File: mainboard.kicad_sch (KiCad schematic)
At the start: 0 parts

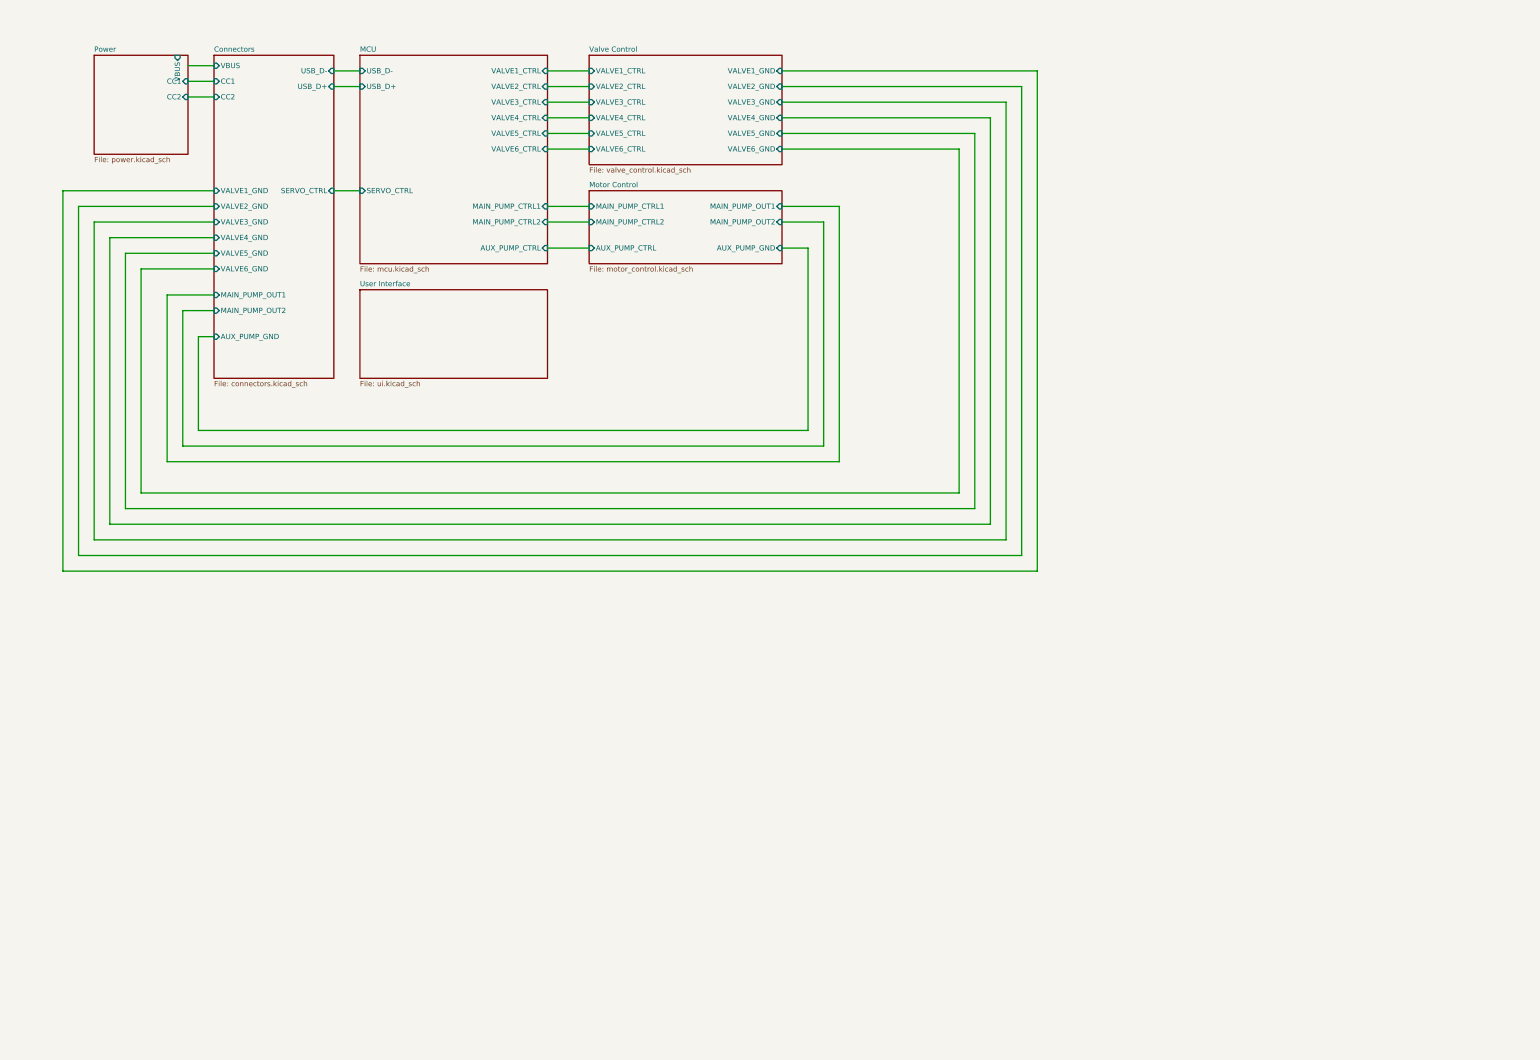
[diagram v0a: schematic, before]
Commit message: Finish first design
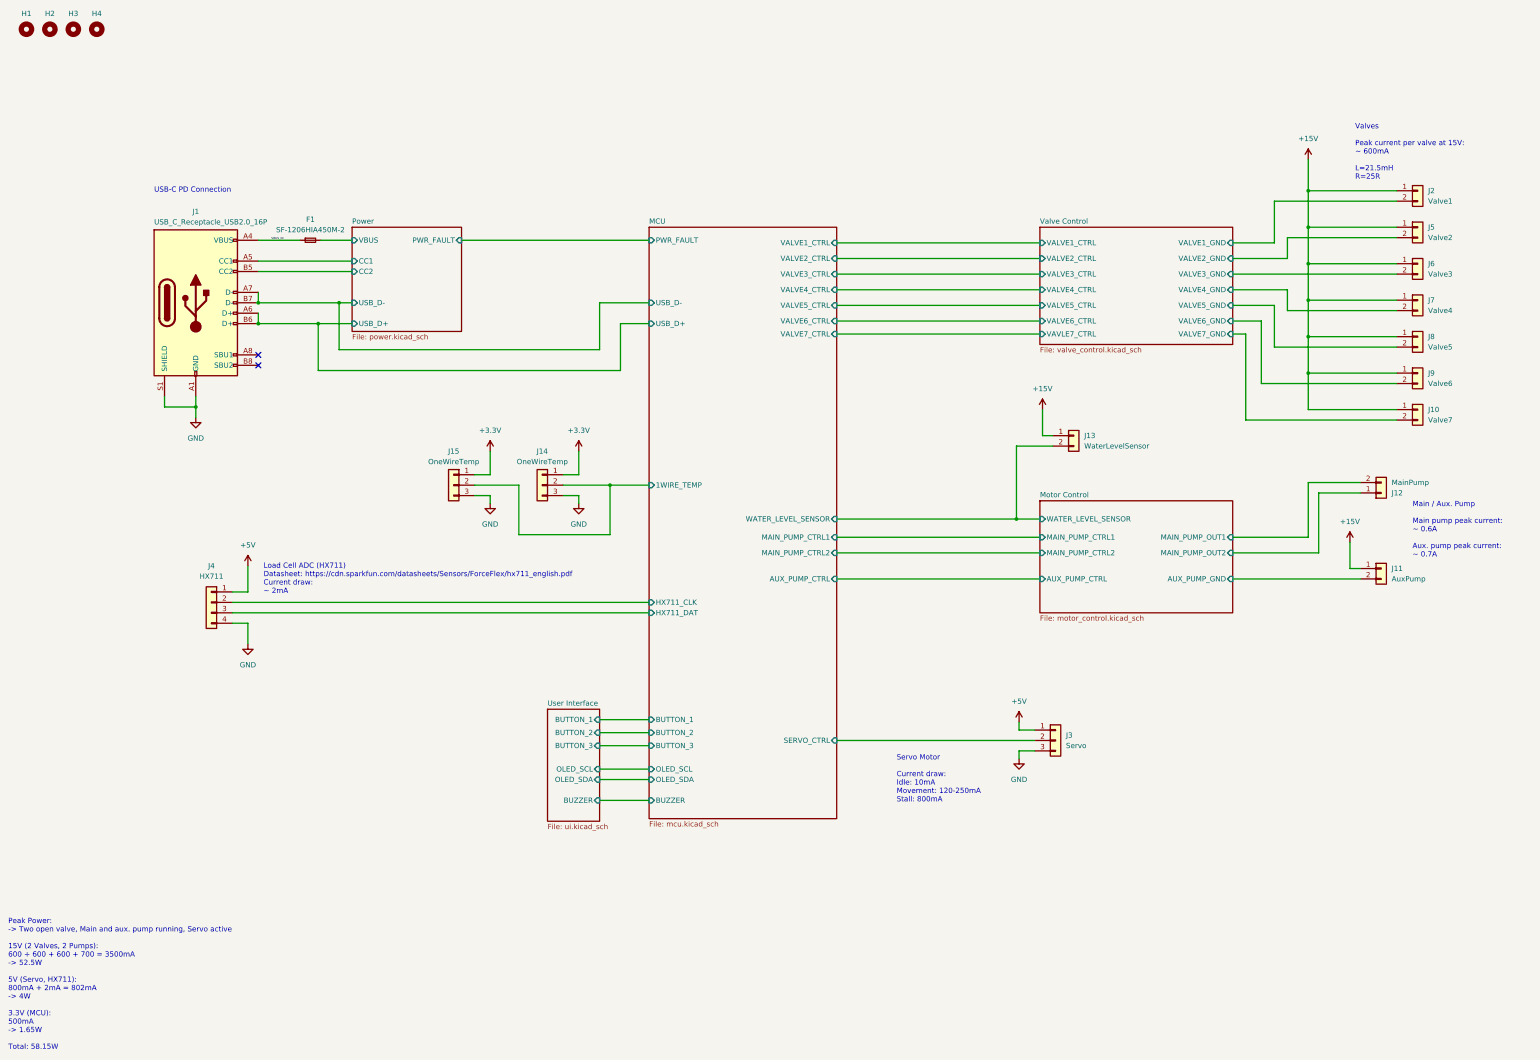
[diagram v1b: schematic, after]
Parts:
- added F1: SF-1206HIA450M-2, Fuse:Fuse_1206_3216Metric, symbol Device:Fuse_Small
- added H1, H2, H3, H4: MountingHole, MountingHole:MountingHole_2.2mm_M2, symbol Mechanical:MountingHole
- added J1: USB_C_Receptacle_USB2.0_16P, project:USB_C_Receptacle_JAE_DX07S016JA1R1500, symbol Connector:USB_C_Receptacle_USB2.0_16P
- added J10: Valve7, Connector_JST:JST_XH_B2B-XH-A_1x02_P2.50mm_Vertical, symbol Connector_Generic:Conn_01x02
- added J11: AuxPump, Connector_JST:JST_XH_B2B-XH-A_1x02_P2.50mm_Vertical, symbol Connector_Generic:Conn_01x02
- added J12: MainPump, Connector_JST:JST_XH_B2B-XH-A_1x02_P2.50mm_Vertical, symbol Connector_Generic:Conn_01x02
- added J13: WaterLevelSensor, Connector_JST:JST_XH_B2B-XH-A_1x02_P2.50mm_Vertical, symbol Connector_Generic:Conn_01x02
- added J14, J15: OneWireTemp, Connector_JST:JST_XH_B3B-XH-A_1x03_P2.50mm_Vertical, symbol Connector_Generic:Conn_01x03
- added J2: Valve1, Connector_JST:JST_XH_B2B-XH-A_1x02_P2.50mm_Vertical, symbol Connector_Generic:Conn_01x02
- added J3: Servo, Connector_JST:JST_XH_B3B-XH-A_1x03_P2.50mm_Vertical, symbol Connector_Generic:Conn_01x03
- added J4: HX711, Connector_JST:JST_XH_B4B-XH-A_1x04_P2.50mm_Vertical, symbol Connector_Generic:Conn_01x04
- added J5: Valve2, Connector_JST:JST_XH_B2B-XH-A_1x02_P2.50mm_Vertical, symbol Connector_Generic:Conn_01x02
- added J6: Valve3, Connector_JST:JST_XH_B2B-XH-A_1x02_P2.50mm_Vertical, symbol Connector_Generic:Conn_01x02
- added J7: Valve4, Connector_JST:JST_XH_B2B-XH-A_1x02_P2.50mm_Vertical, symbol Connector_Generic:Conn_01x02
- added J8: Valve5, Connector_JST:JST_XH_B2B-XH-A_1x02_P2.50mm_Vertical, symbol Connector_Generic:Conn_01x02
- added J9: Valve6, Connector_JST:JST_XH_B2B-XH-A_1x02_P2.50mm_Vertical, symbol Connector_Generic:Conn_01x02
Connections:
- net Power/VBUS: now also F1.2
- new net +15V: J10.1 (Pin_1), J11.1 (Pin_1), J13.1 (Pin_1), J2.1 (Pin_1), J5.1 (Pin_1), J6.1 (Pin_1), J7.1 (Pin_1), J8.1 (Pin_1), J9.1 (Pin_1)
- new net +3.3V: J14.1 (Pin_1), J15.1 (Pin_1)
- new net +5V: J3.1 (Pin_1), J4.1 (Pin_1)
- new net GND: J1.A1 (GND), J1.A12 (GND), J1.B1 (GND), J1.B12 (GND), J1.S1 (SHIELD), J14.3 (Pin_3), J15.3 (Pin_3), J3.3 (Pin_3), J4.4 (Pin_4)
- new net MCU/1WIRE_TEMP: J14.2 (Pin_2), J15.2 (Pin_2)
- new net MCU/HX711_CLK: J4.2 (Pin_2)
- new net MCU/HX711_DAT: J4.3 (Pin_3)
- new net MCU/SERVO_CTRL: J3.2 (Pin_2)
- new net MCU/USB_D+: J1.A6 (D+), J1.B6 (D+)
- new net MCU/USB_D-: J1.A7 (D-), J1.B7 (D-)
- new net MCU/WATER_LEVEL_SENSOR: J13.2 (Pin_2)
- new net Motor Control/AUX_PUMP_GND: J11.2 (Pin_2)
- new net Motor Control/MAIN_PUMP_OUT1: J12.2 (Pin_2)
- new net Motor Control/MAIN_PUMP_OUT2: J12.1 (Pin_1)
- new net Power/CC1: J1.A5 (CC1)
- new net Power/CC2: J1.B5 (CC2)
- new net VBUS_IN: F1.1, J1.A4 (VBUS), J1.A9 (VBUS), J1.B4 (VBUS), J1.B9 (VBUS)
- new net Valve Control/VALVE1_GND: J2.2 (Pin_2)
- new net Valve Control/VALVE2_GND: J5.2 (Pin_2)
- new net Valve Control/VALVE3_GND: J6.2 (Pin_2)
- new net Valve Control/VALVE4_GND: J7.2 (Pin_2)
- new net Valve Control/VALVE5_GND: J8.2 (Pin_2)
- new net Valve Control/VALVE6_GND: J9.2 (Pin_2)
- new net Valve Control/VALVE7_GND: J10.2 (Pin_2)
- no-connect marks 0 -> 2
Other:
- removed sheet Connectors
- sheet MCU ports: added 1WIRE_TEMP, BUTTON_1, BUTTON_2, BUTTON_3, BUZZER, HX711_CLK, HX711_DAT, OLED_SCL, OLED_SDA, PWR_FAULT, VALVE7_CTRL, WATER_LEVEL_SENSOR; removed none
- sheet Motor Control ports: added WATER_LEVEL_SENSOR; removed none
- sheet Power ports: added PWR_FAULT, USB_D+, USB_D-; removed none
- sheet User Interface ports: added BUTTON_1, BUTTON_2, BUTTON_3, BUZZER, OLED_SCL, OLED_SDA; removed none
- sheet Valve Control ports: added VALVE7_GND, VAVLE7_CTRL; removed none
- note added: "Load Cell ADC (HX711) Datasheet: https://cdn.sparkfun.com/datasheets/Sensors/ForceFlex/hx711_english.pdf Current draw: ~ 2mA"
- note added: "Main / Aux. Pump Main pump peak current: ~ 0.6A Aux. pump peak current: ~ 0.7A"
- note added: "Peak Power: -> Two open valve, Main and aux. pump running, Servo active 15V (2 Valves, 2 Pumps): 600 + 600 + 600 + 700 = 3500mA -> 52.5W 5V (Servo, HX711): 800mA + 2mA = 802mA -> 4W 3.3V (MCU): 500mA -> 1.65W Total: 58.15W"
- note added: "Servo Motor Current draw: Idle: 10mA Movement: 120-250mA Stall: 800mA"
- note added: "USB-C PD Connection"
- note added: "Valves Peak current per valve at 15V: ~ 600mA L=21.5mH R=25R"
